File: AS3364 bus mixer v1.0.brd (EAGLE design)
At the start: 41.3 x 16.2 mm, 63 parts, among them IC1 TL072JD, IC2 TL072JD, IC3 TL072JD, IC30 TL072JT, IC4 TL072JD, IC5 79L09F, IC6 78L09F, IC7 CH446Q

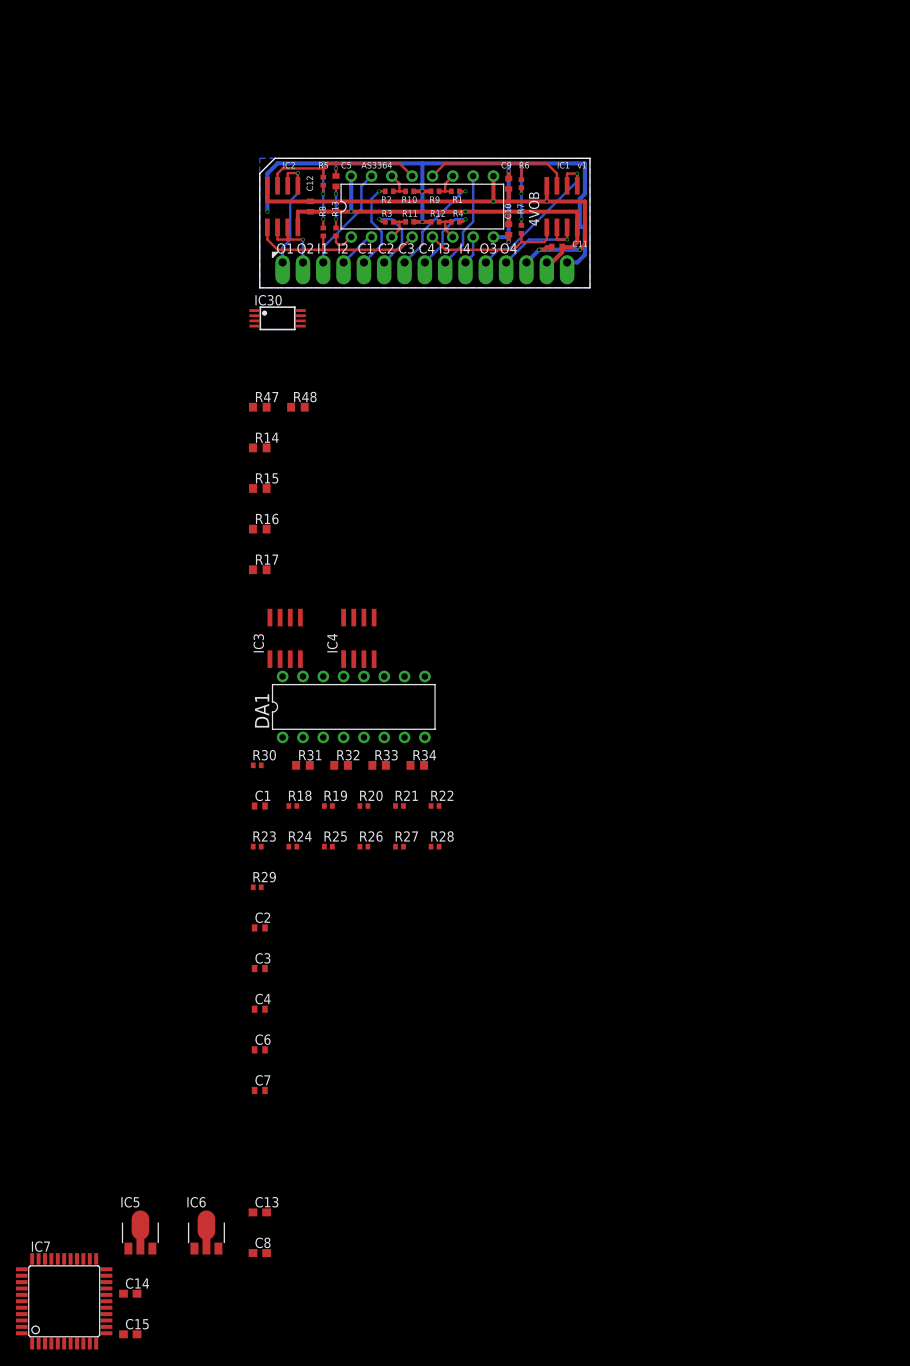
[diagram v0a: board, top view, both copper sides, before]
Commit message: Tracing the bus mixer
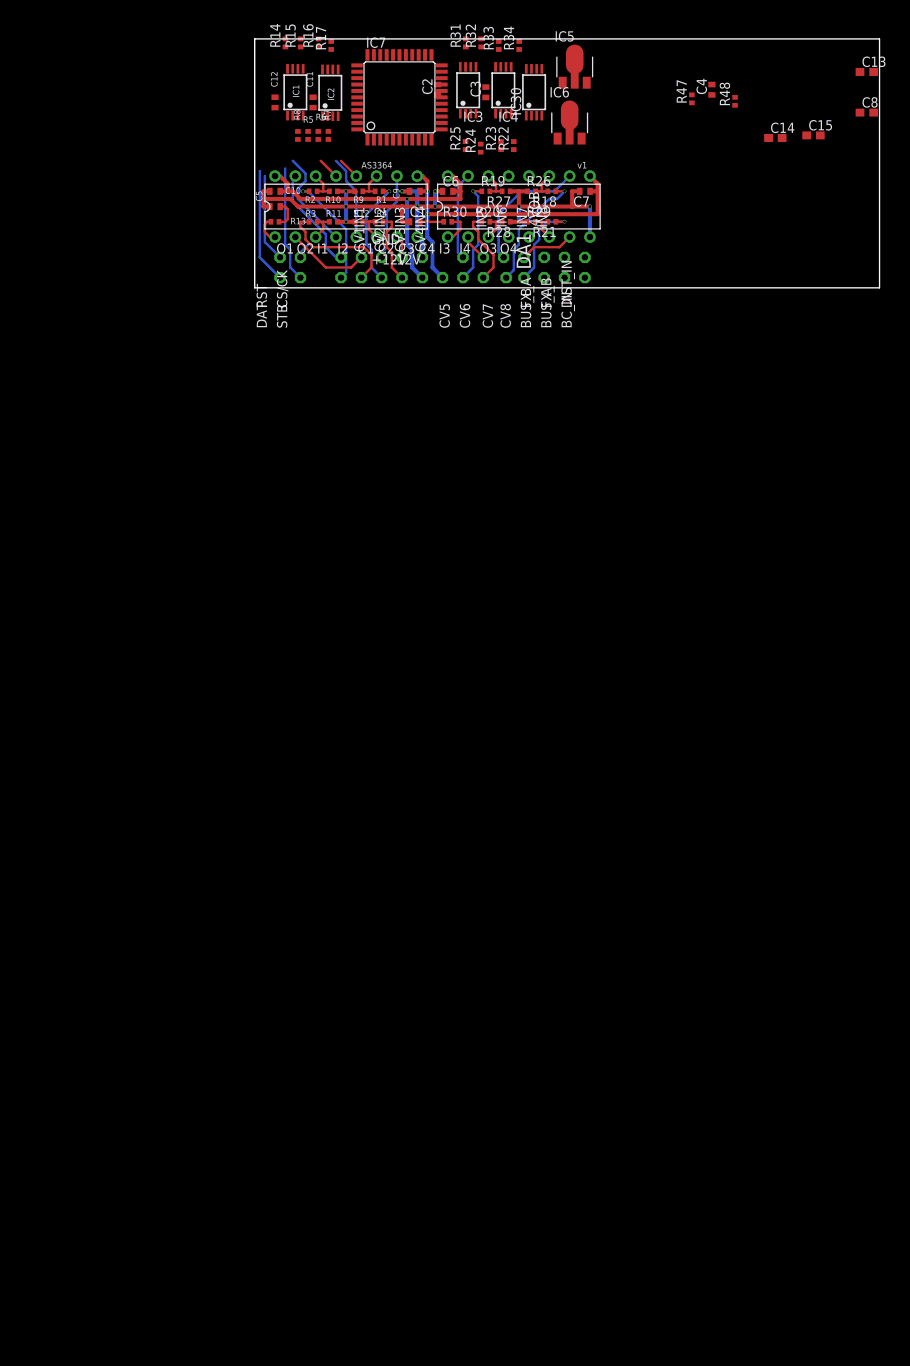
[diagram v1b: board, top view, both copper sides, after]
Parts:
- removed SV1: (no value), joakim:SIP-PIN15-1J
- added +12V, -12V, BC_IN, BUS_A, BUS_B, CS/CK, CV1, CV2, CV3, CV4, CV5, CV6, CV7, CV8, DAT, DIST_IN, FX_A, FX_B, GND, IN1, IN2, IN3, IN4, IN5, IN6, IN7, IN8, RST, STB: (no value), joakim:MA01NS-1J
- IC1, IC2, IC3, IC4: value TL072JD -> TL072JT; device joakim:SO08J -> joakim:TSSOP8J
- R14, R15, R16, R17, R31, R32, R33, R34, R47, R48: device rcl:R0603 -> rcl:R0402
- moved C15 172.5 mm to (69.2, 19.1)
- moved C14 165.4 mm to (64.5, 18.7)
- moved C13 161.5 mm to (75.9, 27.0)
- moved C8 161.5 mm to (75.9, 21.9)
- moved IC7 156.2 mm to (17.5, 23.8)
- moved IC5 155.5 mm to (39.4, 27.6)
- moved IC6 146.0 mm to (38.7, 20.6)
- moved C4 128.1 mm to (56.5, 24.8), turned to 90 degrees
- moved C7 119.5 mm to (40.6, 12.1), turned to 180 degrees
- moved C3 113.1 mm to (28.3, 24.4), turned to 90 degrees
- moved C6 109.9 mm to (23.5, 12.1)
- moved C2 107.1 mm to (22.2, 24.8), turned to 90 degrees
- moved R23 92.8 mm to (30.2, 17.8), turned to 90 degrees
- moved R31 92.6 mm to (25.8, 30.6), turned to 90 degrees
- moved R32 92.0 mm to (27.7, 30.6), turned to 90 degrees
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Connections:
- new net BITCRUSH_IN: BC_IN.1, IC7.15
- new net CS/CK: CS/CK.1, IC7.34
- new net CV5: CV5.1, R19.1
- new net CV6: CV6.1, R20.1
- new net CV6_IN: DA1.3, R20.2, R28.2
- new net CV7: CV7.1, R18.1
- new net CV8: CV8.1, R21.1
- new net DAT: DAT.1, IC7.36
- new net DIST_IN: DIST_IN.1, IC7.17
- new net FX_A: FX_A.1, IC7.37
- new net FX_B: FX_B.1, IC7.39
- new net IN5: DA1.15, IN5.1
- new net IN6: DA1.2, IN6.1
- new net IN7: DA1.10, IN7.1
- new net IN8: DA1.7, IN8.1
- new net OUT5: IC4.1, IC4.2, R34.1
- new net OUT6: IC4.6, IC4.7, R31.1
- new net OUT7: IC3.1, IC3.2, R33.1
- new net OUT8: IC3.6, IC3.7, R32.1
- new net RST: IC7.41, RST.1
- new net STB: IC7.14, STB.1
- new net SW1: IC7.31, R17.2
- new net SW2: IC7.30, R14.2
- new net SW3: IC7.29, R16.2
- new net SW4: IC7.28, R15.2
- new net SW5: IC7.27, R34.2
- new net SW6: IC7.26, R31.2
- new net SW7: IC7.3, R33.2
- new net SW8: IC7.4, R32.2
- net +12V: now also +12V.1; no longer SV1.14
- net -12V: now also -12V.1; no longer SV1.13
- net BUS_A: now also BUS_A.1, IC7.33
- net BUS_B: now also BUS_B.1, IC7.35
- net CV1: now also CV1.1; no longer R19.1, SV1.5
- net CV2: now also CV2.1; no longer R20.1, SV1.6
- net CV2_IN: no longer DA1.3, R20.2, R28.2
- net CV3: now also CV3.1; no longer R18.1, SV1.7
- net CV4: now also CV4.1; no longer R21.1, SV1.8
- net GND: now also GND.1; no longer SV1.15
- net IN1: now also IN1.1; no longer DA1.15, SV1.3
- net IN2: now also IN2.1; no longer DA1.2, SV1.4
- net IN3: now also IN3.1; no longer DA1.10, SV1.9
- net IN4: now also IN4.1; no longer DA1.7, SV1.10
- net OUT1: no longer IC4.1, IC4.2, R34.1, SV1.1
- net OUT2: no longer IC4.6, IC4.7, R31.1, SV1.2
- net OUT3: no longer IC3.1, IC3.2, R33.1, SV1.11
- net OUT4: no longer IC3.6, IC3.7, R32.1, SV1.12
- net SUM_A: now also IC30.7, IC7.5, R47.2; no longer IC30.1, R48.2
- net SUM_B: now also IC30.1, IC7.6, R48.2; no longer IC30.7, R47.2
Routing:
- net -12V: track 63.7 -> 42.7 mm, vias 4 -> 2
- net OUT3: track 20.9 -> 0.00 mm, vias 1 -> 0
- net GND: track 104.5 -> 84.7 mm
- net N$13: track 20.6 -> 2.69 mm
- net N$11: track 20.3 -> 2.69 mm
- net IN7: track 0.00 -> 16.5 mm
- net OUT1: track 16.4 -> 0.00 mm, vias 1 -> 0
- net CV7: track 0.00 -> 15.5 mm, vias 0 -> 1
- net STB: track 0.00 -> 14.4 mm
- net DAT: track 0.00 -> 14.4 mm
- net OUT4: track 13.1 -> 0.00 mm, vias 1 -> 0
- net CV5: track 0.00 -> 12.9 mm, vias 0 -> 1
- net CV8: track 0.00 -> 11.5 mm, vias 0 -> 1
- net RST: track 0.00 -> 10.9 mm
- net IN5: track 0.00 -> 10.9 mm
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- removed copper zone on layer 16, net GND
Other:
- board size 41.3 x 16.2 mm -> 78.1 x 31.1 mm
